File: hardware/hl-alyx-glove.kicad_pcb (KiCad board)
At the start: 2 copper layers, 20 parts, among them J1 OLED, J2 POWER, U1 MAX7219, U2 MAX7219, U3 MAX7219, U4 ATmega328P-PU

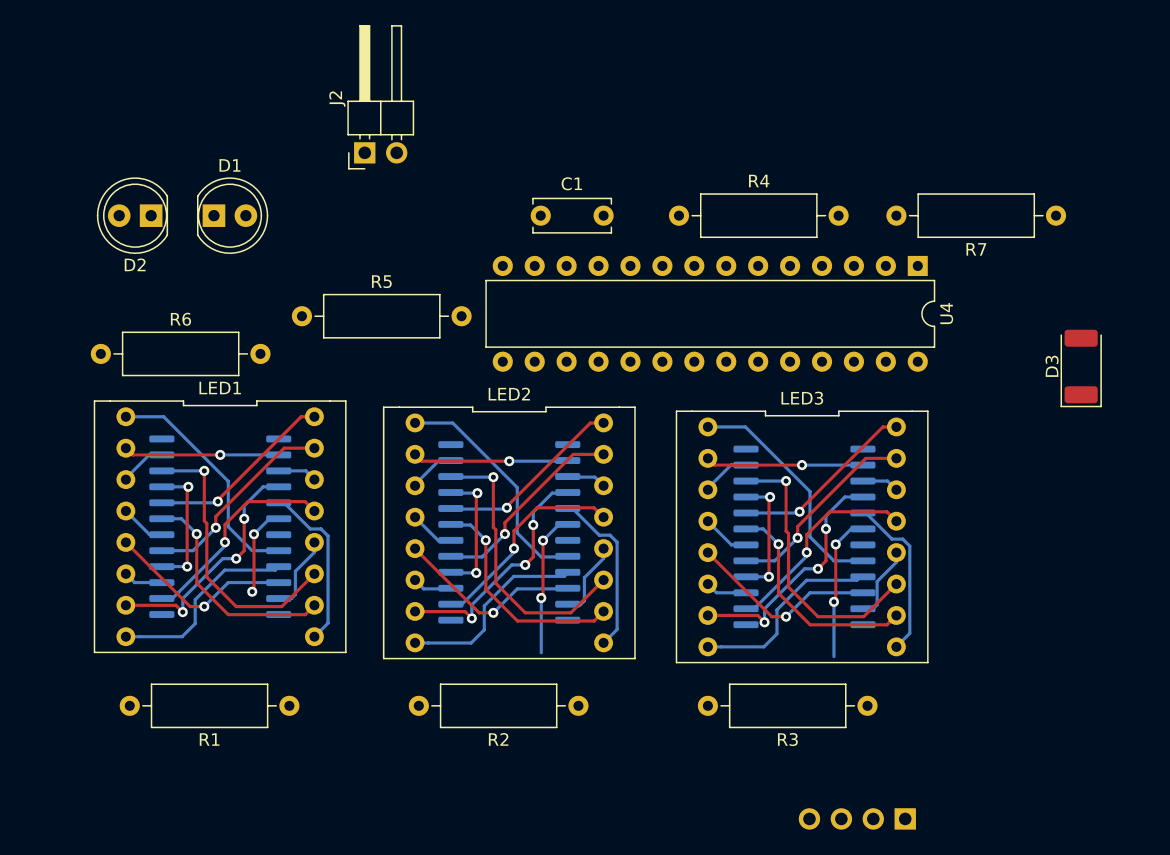
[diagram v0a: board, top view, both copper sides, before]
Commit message: pcb first version
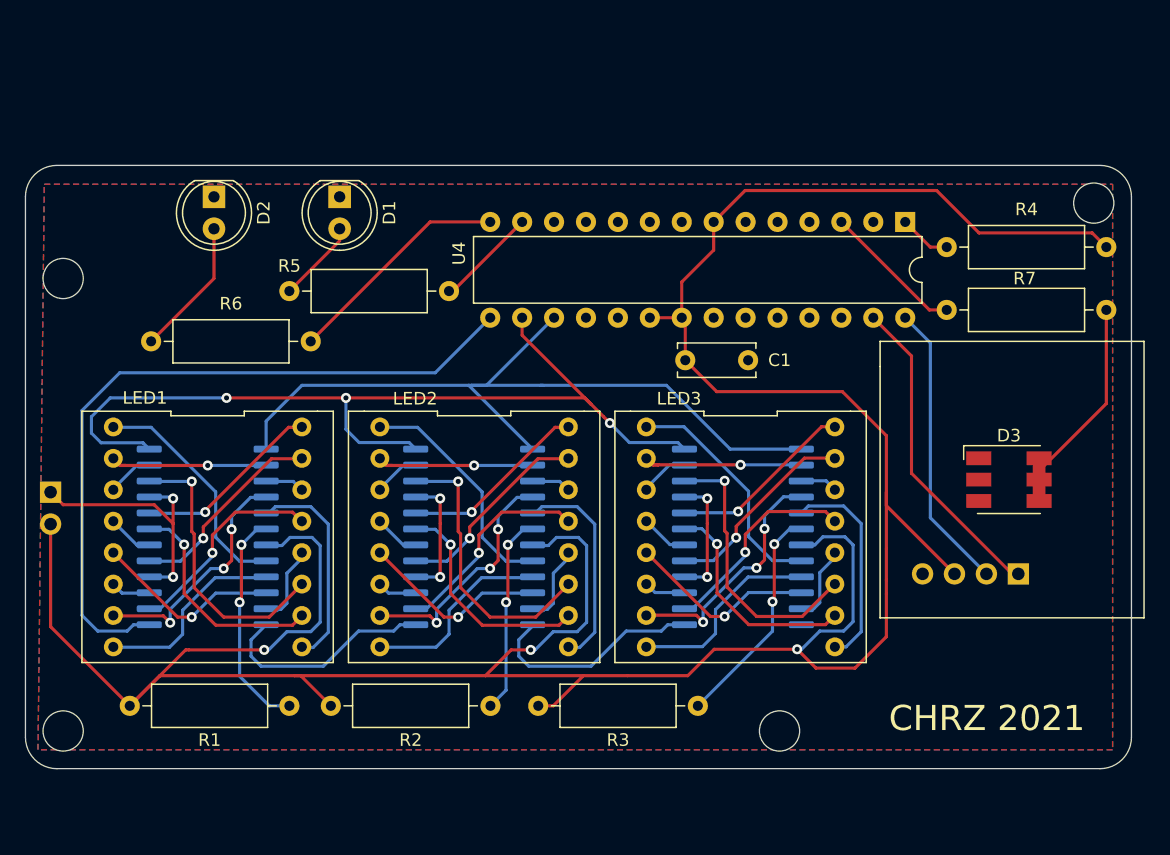
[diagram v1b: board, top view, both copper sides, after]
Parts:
- added REF**: MountingHole_3.2mm_M3, MountingHole:MountingHole_3.2mm_M3, F.Cu at (88.0, 90.0)
- added REF**: MountingHole_3.2mm_M3, MountingHole:MountingHole_3.2mm_M3, F.Cu at (88.0, 54.0)
- added REF**: MountingHole_3.2mm_M3, MountingHole:MountingHole_3.2mm_M3, F.Cu at (170.0, 48.0)
- added REF**: MountingHole_3.2mm_M3, MountingHole:MountingHole_3.2mm_M3, F.Cu at (145.0, 90.0)
- D3: footprint LED_SMD:LED_2010_5025Metric -> LED_SMD:LED_RGB_5050-6
- J2: moved to B.Cu
- R7: value 100 -> 180
- moved J2 36.8 mm to (87.0, 71.0), turned to 180 degrees
- moved R4 34.1 mm to (171.0, 51.5), turned to 180 degrees
- moved J1 21.5 mm to (164.0, 77.5)
- moved C1 16.3 mm to (137.5, 60.5)
- moved R3 13.5 mm to (138.5, 88.0)
- moved D3 10.7 mm to (163.2, 70.0), turned to 0 degrees
- moved D1 10.1 mm to (110.0, 47.5), turned to 270 degrees
- moved R7 8.50 mm to (171.0, 56.5)
- moved R2 7.00 mm to (122.0, 88.0)
- moved D2 5.22 mm to (100.0, 47.5), turned to 270 degrees
- moved U3 4.90 mm to (142.1, 74.6)
- moved LED3 4.90 mm to (141.9, 74.6)
- moved R6 4.12 mm to (95.0, 59.0)
- moved U4 3.64 mm to (155.0, 49.5)
- moved U2 2.82 mm to (120.7, 74.6)
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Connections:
- D3 pad 2: Net-(D3-Pad2) -> GND
- J2 pad 1: +3V3 -> GND
- J2 pad 2: GND -> +3V3
- R7 pad 1: Net-(D3-Pad2) -> Net-(D3-Pad4)
- U4 pad 11: Net-(R6-Pad2) -> Net-(U4-Pad11)
- U4 pad 12: Net-(R5-Pad2) -> Net-(U4-Pad12)
- U4 pad 13: Net-(R7-Pad2) -> Net-(R5-Pad2)
- U4 pad 14: Net-(U4-Pad14) -> Net-(R6-Pad2)
- U4 pad 15: Net-(U4-Pad15) -> /LED_Matrix_0/DIN
- U4 pad 18: /LED_Matrix_0/DIN -> Net-(U4-Pad18)
- U4 pad 3: Net-(U4-Pad3) -> Net-(R7-Pad2)
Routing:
- net +3V3: track 0.00 -> 246.7 mm, vias 0 -> 3
- net /LED_Matrix_0/LOAD: track 0.00 -> 74.6 mm, vias 0 -> 3
- net /LED_Matrix_0/CLK: track 0.00 -> 64.2 mm
- net /LED_Matrix_0/DIN: track 0.00 -> 57.9 mm
- net Net-(J1-Pad1): track 0.00 -> 25.5 mm
- net Net-(J1-Pad2): track 0.00 -> 23.1 mm
- net Net-(D3-Pad4): track 0.00 -> 18.6 mm
- net Net-(R6-Pad2): track 0.00 -> 18.2 mm
- net /LED_Matrix_1/DIN: track 0.00 -> 17.8 mm
- net /LED_Matrix_2/DIN: track 0.00 -> 17.8 mm
- net Net-(R7-Pad2): track 0.00 -> 11.3 mm
- net Net-(D2-Pad2): track 0.00 -> 11.0 mm
- net Net-(R1-Pad1): track 7.11 -> 17.9 mm
- net GND: track 31.6 -> 40.7 mm
- net Net-(R5-Pad2): track 0.00 -> 8.10 mm
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- added copper zone on B.Cu, net GND
- added copper zone on F.Cu, net GND
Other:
- board outline added: 88 x 48 mm
- board text added: "CHRZ 2021"
